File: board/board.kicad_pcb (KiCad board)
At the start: 2 copper layers, 21 x 13 mm, 1 part

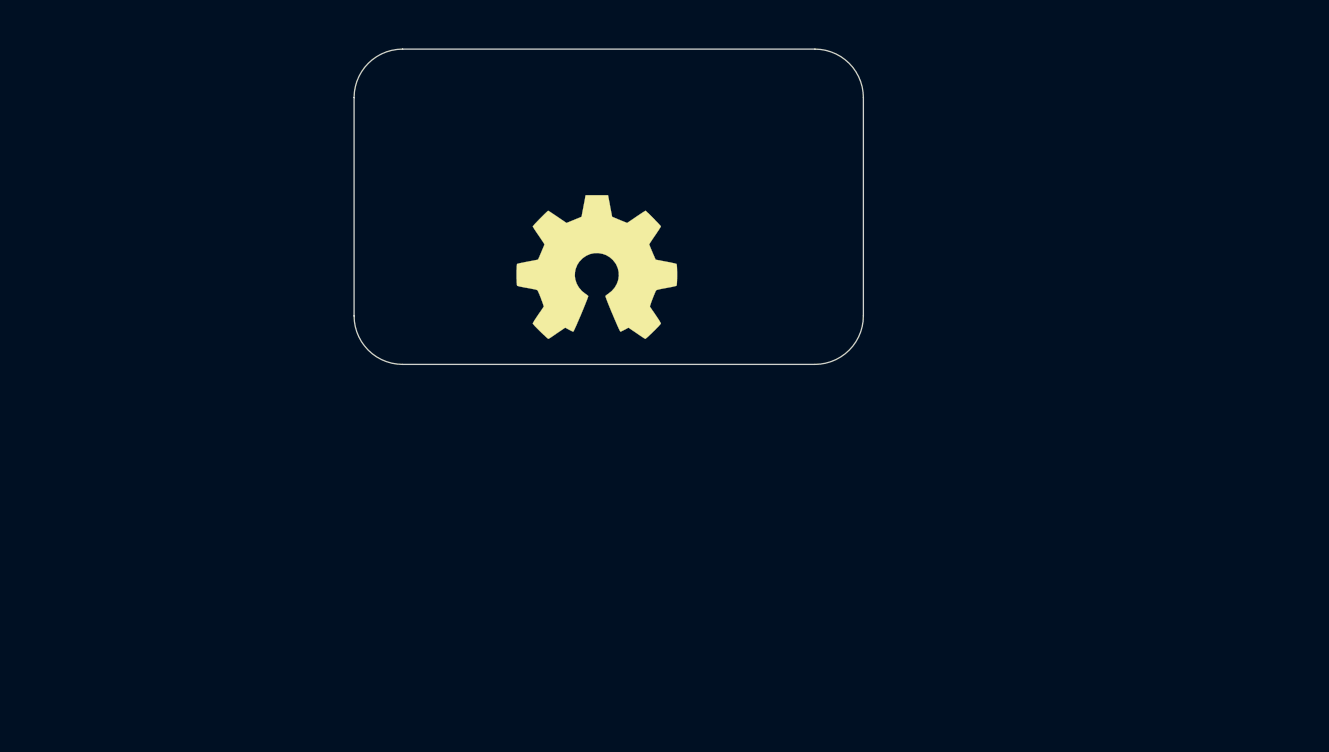
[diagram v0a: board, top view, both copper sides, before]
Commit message: initial hw
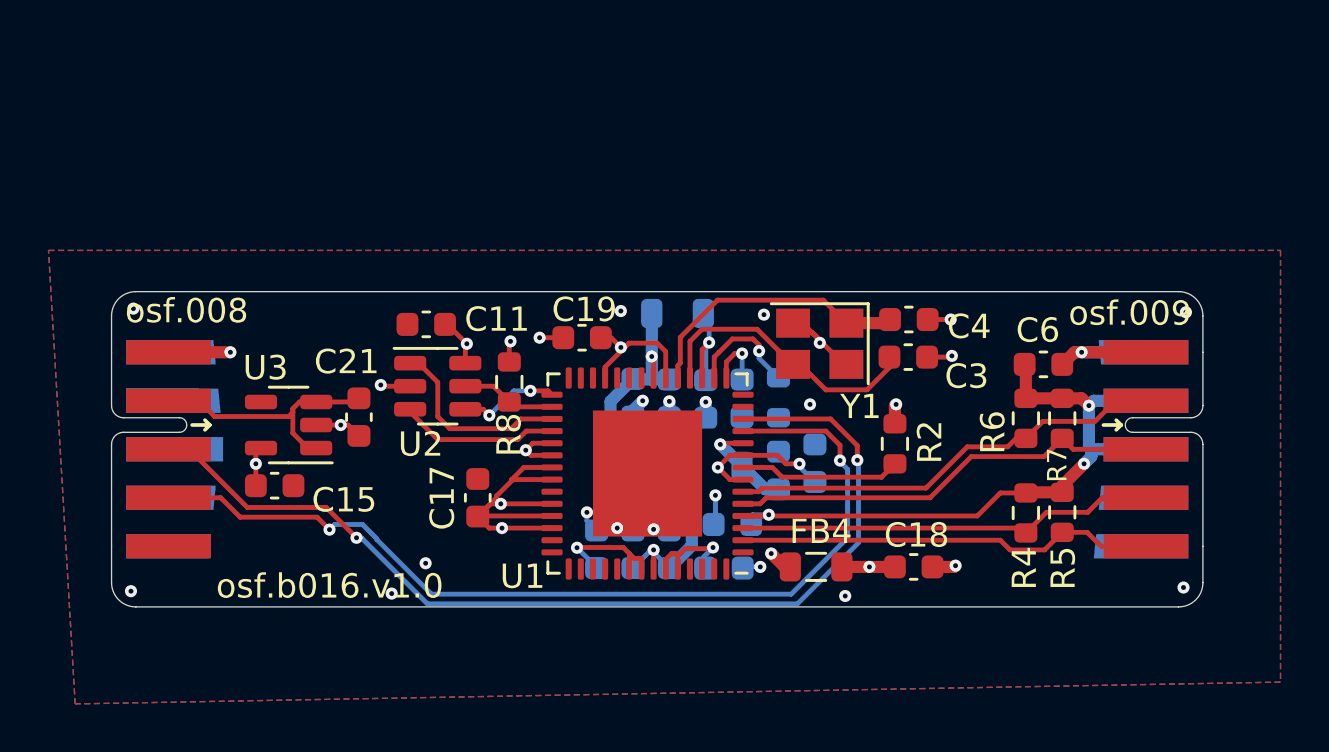
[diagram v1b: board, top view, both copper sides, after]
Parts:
- removed LOGO1: Logo_Open_Hardware_Small, Symbol:OSHW-Symbol_6.7x6mm_SilkScreen
- added C1: 1uF, Capacitor_SMD:C_0603_1608Metric, B.Cu at (153.0, 110.6)
- added C10: 100nF, Capacitor_SMD:C_0603_1608Metric, B.Cu at (150.0, 110.6)
- added C11: 100nF, Capacitor_SMD:C_0603_1608Metric, F.Cu at (143.0, 101.3)
- added C12: 100nF, Capacitor_SMD:C_0603_1608Metric, B.Cu at (156.0, 104.4)
- added C13: 100nF, Capacitor_SMD:C_0603_1608Metric, B.Cu at (155.2, 111.4)
- added C14: 100nF, Capacitor_SMD:C_0603_1608Metric, B.Cu at (155.6, 109.6)
- added C15: 4.7nF, Capacitor_SMD:C_0603_1608Metric, F.Cu at (136.7, 108.0)
- added C16: 4.7nF, Capacitor_SMD:C_0603_1608Metric, B.Cu at (159.0, 107.1)
- added C17: 4.7nF, Capacitor_SMD:C_0603_1608Metric, F.Cu at (145.1, 108.5)
- added C18: 1.5nF, Capacitor_SMD:C_0603_1608Metric, F.Cu at (163.1, 111.3)
- added C19: 1.5nF, Capacitor_SMD:C_0603_1608Metric, F.Cu at (149.4, 101.9)
- added C2: 100nF, Capacitor_SMD:C_0603_1608Metric, B.Cu at (153.0, 104.4)
- added C21: 1uF, Capacitor_SMD:C_0603_1608Metric, F.Cu at (140.2, 105.2)
- added C3: 10pF, Capacitor_SMD:C_0603_1608Metric, F.Cu at (162.8, 102.7)
- added C4: 10pF, Capacitor_SMD:C_0603_1608Metric, F.Cu at (162.9, 101.2)
- added C5: 4.7nF, Capacitor_SMD:C_0603_1608Metric, B.Cu at (151.5, 104.4)
- added C6: 100nF, Capacitor_SMD:C_0603_1608Metric, F.Cu at (168.4, 103.0)
- added C7: 4.7nF, Capacitor_SMD:C_0603_1608Metric, B.Cu at (157.5, 107.4)
- added C8: 4.7nF, Capacitor_SMD:C_0603_1608Metric, B.Cu at (154.5, 104.4)
- added C9: 1.5nF, Capacitor_SMD:C_0603_1608Metric, B.Cu at (151.5, 110.6)
- added FB2: 220R, Inductor_SMD:L_0805_2012Metric, B.Cu at (154.9, 107.2)
- added FB3: 220R, Inductor_SMD:L_0805_2012Metric, B.Cu at (153.3, 100.9)
- added FB4: 220R, Inductor_SMD:L_0805_2012Metric, F.Cu at (159.1, 111.3)
- added J1: 008_USB_2x2, on_edge:on_edge_2x05_device, F.Cu at (130.0, 106.5)
- added J2: 009_1000BASE-T_2x5, on_edge:on_edge_2x05_host, F.Cu at (175.0, 106.5)
- added R2: 12k, Resistor_SMD:R_0603_1608Metric, F.Cu at (162.3, 106.3)
- added R3: 12k, Resistor_SMD:R_0603_1608Metric, B.Cu at (157.5, 104.4)
- added R4: 49.9R, Resistor_SMD:R_0603_1608Metric, F.Cu at (167.7, 109.1)
- added R5: 49.9R, Resistor_SMD:R_0603_1608Metric, F.Cu at (169.2, 109.1)
- added R6: 49.9R, Resistor_SMD:R_0603_1608Metric, F.Cu at (167.7, 105.2)
- added R7: 49.9R, Resistor_SMD:R_0603_1608Metric, F.Cu at (169.2, 105.2)
- added R8: 12k, Resistor_SMD:R_0603_1608Metric, F.Cu at (146.4, 103.7)
- added U1: LAN9500(A), Package_DFN_QFN:QFN-56-1EP_8x8mm_P0.5mm_EP4.5x5.2mm, F.Cu at (152.1, 107.5)
- added U2: 93AA56AT-I/OT, Package_TO_SOT_SMD:SOT-23-6, F.Cu at (143.4, 103.9)
- added U3: TC1017-xCT, Package_TO_SOT_SMD:SOT-23-5, F.Cu at (137.3, 105.5)
- added Y1: 25MhZ, Crystal:Crystal_SMD_Abracon_ABM8G-4Pin_3.2x2.5mm, F.Cu at (159.2, 102.2)
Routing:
- net /Sheet603703E3/CT1: track 0.00 -> 49.5 mm, vias 0 -> 7
- net GND: track 0.00 -> 41.9 mm, vias 0 -> 30
- net /Sheet603703E3/DP: track 0.00 -> 41.3 mm, vias 0 -> 2
- net /Sheet603703E3/DM: track 0.00 -> 39.0 mm, vias 0 -> 2
- net +3.3V: track 0.00 -> 37.3 mm, vias 0 -> 8
- net Net-(C1-Pad1): track 0.00 -> 19.1 mm, vias 0 -> 2
- net /Sheet603703E3/D2+: track 0.00 -> 18.2 mm
- net /Sheet603703E3/D2-: track 0.00 -> 17.9 mm
- net /Sheet603703E3/D1-: track 0.00 -> 17.3 mm
- net /Sheet603703E3/D1+: track 0.00 -> 17.3 mm
- net Net-(C3-Pad1): track 0.00 -> 12.2 mm
- net Net-(C4-Pad1): track 0.00 -> 11.5 mm
- net /VCC: track 0.00 -> 10.6 mm
- net Net-(U1-Pad31): track 0.00 -> 7.96 mm
- net Net-(R2-Pad2): track 0.00 -> 6.66 mm
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- added copper zone on In2.Cu, net +3.3V
- added copper zone on In2.Cu, net /Sheet603703E3/CT1
- added copper zone on B.Cu, net GND
- added copper zone on F.Cu, net GND
- added copper zone on In1.Cu, net GND
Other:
- board size 21 x 13 mm -> 45 x 13 mm
- copper layers 2 -> 4
- rule pad_to_mask_clearance: 0 -> 0.051
- board text added: "osf.008"
- board text added: "osf.009"
- board text added: "osf.b016.v1.0"
